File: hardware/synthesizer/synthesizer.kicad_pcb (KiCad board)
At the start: 2 copper layers, 15 parts, among them J1 Conn_ARM_SWD_TagConnect_TC2030, J10 Output 2, J11 RJ45_Abracon_ARJP11A-MASA-B-A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, J6 Input 1, J7 Input 2, J9 Output 1, U1 MAX40200ANS, U2 LAN8742A, U3 AP2112K-1.2, U4 STM32H723VGT6, U5 AP2112K-3.3, U6 USBLC6-2P6, Y2 SG-210STF

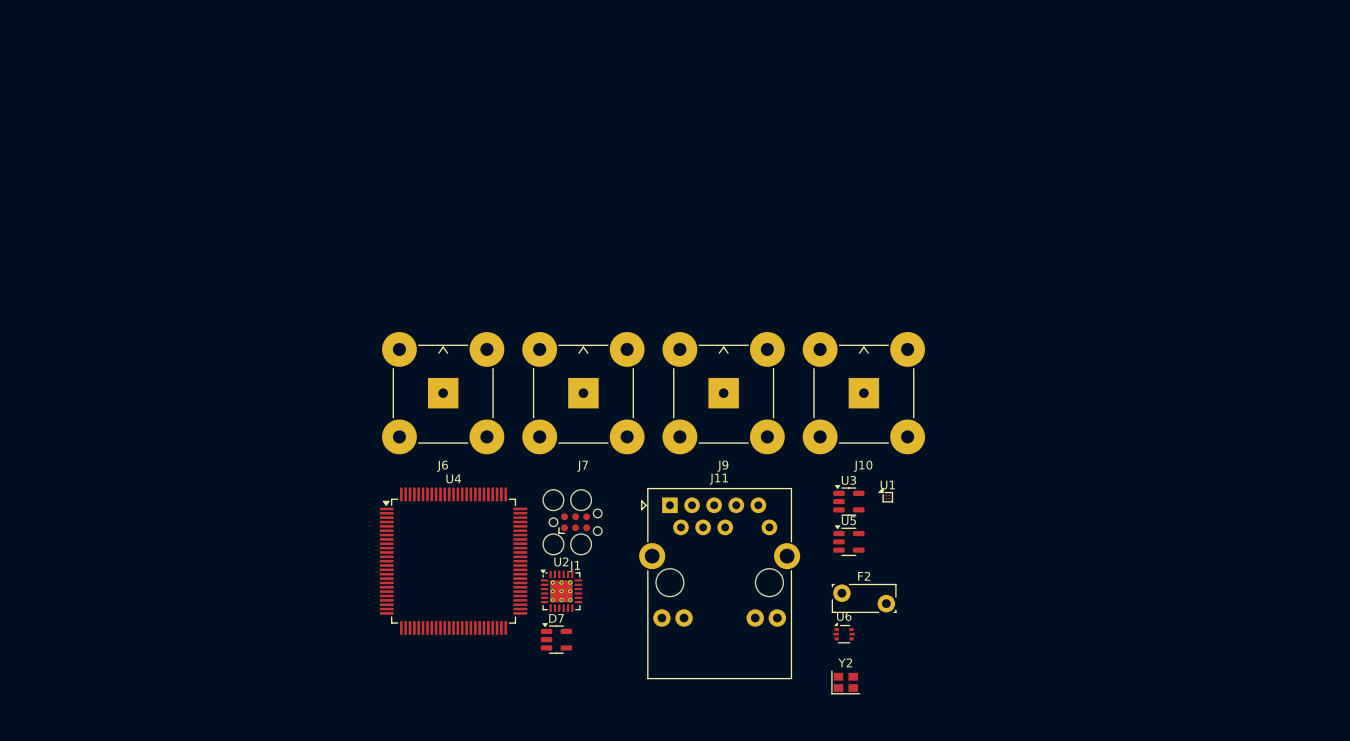
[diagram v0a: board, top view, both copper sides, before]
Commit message: improved pcb design
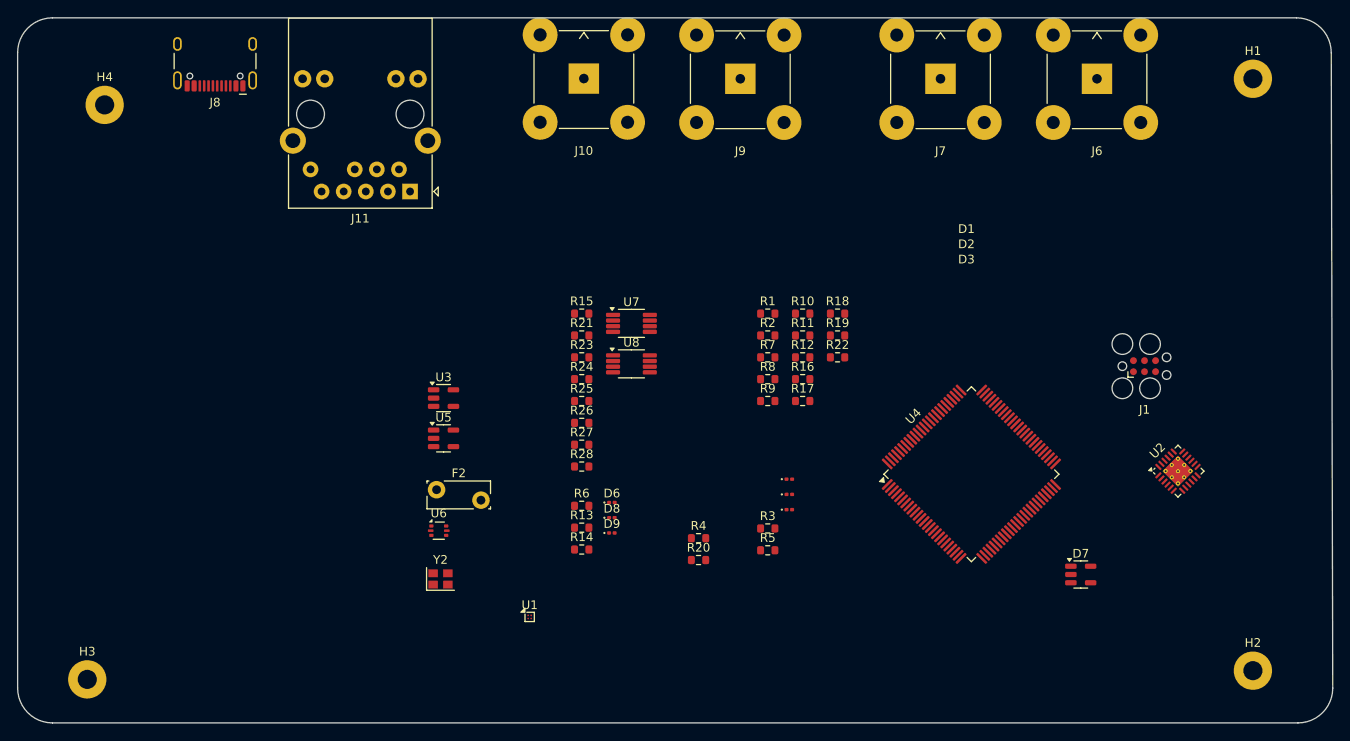
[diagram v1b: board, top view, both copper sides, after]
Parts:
- added D1: Yellow, LED_SMD:LED_0201_0603Metric, F.Cu at (165.7, 93.0)
- added D2: Red, LED_SMD:LED_0201_0603Metric, F.Cu at (165.7, 94.8)
- added D3: Green, LED_SMD:LED_0201_0603Metric, F.Cu at (165.7, 96.5)
- added D6: Red, LED_SMD:LED_0201_0603Metric, F.Cu at (145.3, 95.7)
- added D8: Blue, LED_SMD:LED_0201_0603Metric, F.Cu at (145.3, 97.4)
- added D9: Orange, LED_SMD:LED_0201_0603Metric, F.Cu at (145.3, 99.2)
- added H1: MountingHole, MountingHole:MountingHole_2.2mm_M2_Pad, F.Cu at (218.9, 47.0)
- added H2: MountingHole, MountingHole:MountingHole_2.2mm_M2_Pad, F.Cu at (218.9, 115.0)
- added H3: MountingHole, MountingHole:MountingHole_2.2mm_M2_Pad, F.Cu at (85.0, 116.0)
- added H4: MountingHole, MountingHole:MountingHole_2.2mm_M2_Pad, F.Cu at (87.0, 50.0)
- added J8: USB_C_Receptacle_USB2.0_14P, Connector_USB:USB_C_Receptacle_HCTL_HC-TYPE-C-16P-01A, F.Cu at (99.7, 44.1)
- added R1: 1k, Resistor_SMD:R_0603_1608Metric, F.Cu at (163.2, 74.0)
- added R10: 10k, Resistor_SMD:R_0603_1608Metric, F.Cu at (167.2, 74.0)
- added R11: 10k, Resistor_SMD:R_0603_1608Metric, F.Cu at (167.2, 76.5)
- added R12: 5.6k, Resistor_SMD:R_0603_1608Metric, F.Cu at (167.2, 79.0)
- added R13: 1k, Resistor_SMD:R_0603_1608Metric, F.Cu at (141.8, 98.6)
- added R14: 1k, Resistor_SMD:R_0603_1608Metric, F.Cu at (141.8, 101.1)
- added R15: 200k, Resistor_SMD:R_0603_1608Metric, F.Cu at (141.8, 74.0)
- added R16: 100k, Resistor_SMD:R_0603_1608Metric, F.Cu at (167.2, 81.5)
- added R17: 1k, Resistor_SMD:R_0603_1608Metric, F.Cu at (167.2, 84.0)
- added R18: 10k, Resistor_SMD:R_0603_1608Metric, F.Cu at (171.2, 74.0)
- added R19: 49.9k, Resistor_SMD:R_0603_1608Metric, F.Cu at (171.2, 76.5)
- added R2: 1k, Resistor_SMD:R_0603_1608Metric, F.Cu at (163.2, 76.5)
- added R20: 470, Resistor_SMD:R_0603_1608Metric, F.Cu at (155.2, 102.3)
- added R21: 10k, Resistor_SMD:R_0603_1608Metric, F.Cu at (141.8, 76.5)
- added R22: 10k, Resistor_SMD:R_0603_1608Metric, F.Cu at (171.2, 79.0)
- added R23: 200k, Resistor_SMD:R_0603_1608Metric, F.Cu at (141.8, 79.0)
- added R24: 6.8k, Resistor_SMD:R_0603_1608Metric, F.Cu at (141.8, 81.5)
- added R25: 10k, Resistor_SMD:R_0603_1608Metric, F.Cu at (141.8, 84.0)
- added R26: 200k, Resistor_SMD:R_0603_1608Metric, F.Cu at (141.8, 86.5)
- added R27: 4.7k, Resistor_SMD:R_0603_1608Metric, F.Cu at (141.8, 89.0)
- added R28: 10k, Resistor_SMD:R_0603_1608Metric, F.Cu at (141.8, 91.5)
- added R3: 5.1k, Resistor_SMD:R_0603_1608Metric, F.Cu at (163.2, 98.7)
- added R4: 470, Resistor_SMD:R_0603_1608Metric, F.Cu at (155.2, 99.8)
- added R5: 5.1k, Resistor_SMD:R_0603_1608Metric, F.Cu at (163.2, 101.2)
- added R6: 1k, Resistor_SMD:R_0603_1608Metric, F.Cu at (141.8, 96.1)
- added R7: 49.9k, Resistor_SMD:R_0603_1608Metric, F.Cu at (163.2, 79.0)
- added R8: 49.9k, Resistor_SMD:R_0603_1608Metric, F.Cu at (163.2, 81.5)
- added R9: 49.9k, Resistor_SMD:R_0603_1608Metric, F.Cu at (163.2, 84.0)
- added U7: OPA196xDGK, Package_SO:VSSOP-8_3x3mm_P0.65mm, F.Cu at (147.5, 75.1)
- added U8: OPA196xDGK, Package_SO:VSSOP-8_3x3mm_P0.65mm, F.Cu at (147.5, 79.8)
- moved J6 83.3 mm to (201.0, 47.0)
- moved U2 72.2 mm to (210.3, 92.1), turned to 45 degrees
- moved J1 67.8 mm to (206.5, 80.0)
- moved D7 60.7 mm to (199.1, 104.0)
- moved U4 60.3 mm to (186.6, 92.4), turned to 45 degrees
- moved J7 54.7 mm to (183.0, 47.0)
- moved J10 48.4 mm to (142.1, 47.0)
- moved Y2 48.1 mm to (125.6, 104.5)
- moved F2 48.1 mm to (125.1, 94.2)
- moved U3 48.1 mm to (125.9, 83.7)
- moved U5 48.1 mm to (125.9, 88.3)
- moved U6 48.1 mm to (125.4, 98.9)
- moved J11 46.8 mm to (122.1, 60.0), turned to 180 degrees
- moved U1 43.4 mm to (135.8, 108.8)
- moved J9 36.2 mm to (160.0, 47.0)
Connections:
- J10 pad 1: unconnected-(J10-In-Pad1) -> /Coxial Connectors/OUT_2
- J6 pad 1: unconnected-(J6-In-Pad1) -> /Coxial Connectors/IN_1
- J7 pad 1: unconnected-(J7-In-Pad1) -> /Coxial Connectors/IN_2
- J9 pad 1: unconnected-(J9-In-Pad1) -> /Coxial Connectors/OUT_1
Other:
- board outline added: 151.1 x 81 mm
